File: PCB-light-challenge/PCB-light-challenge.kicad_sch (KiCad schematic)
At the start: 2 parts

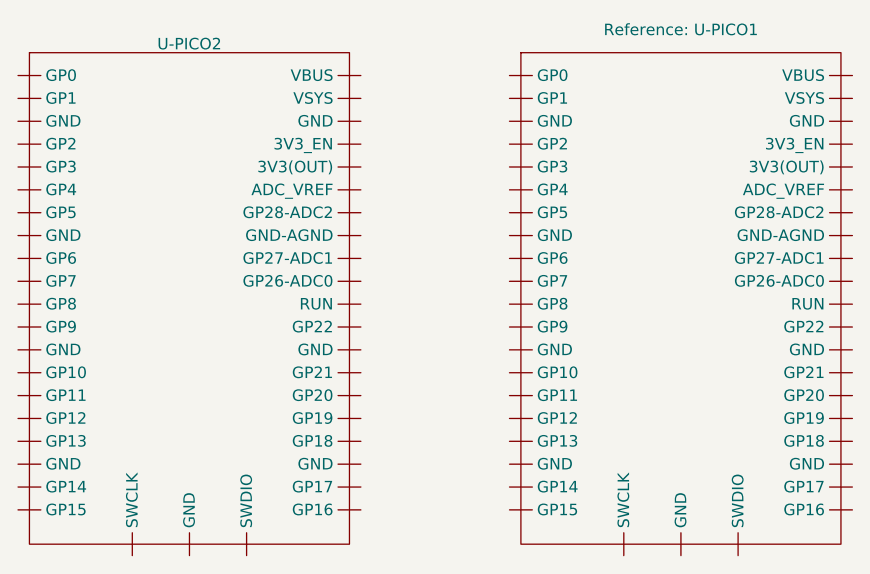
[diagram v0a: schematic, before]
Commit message: Opnieuw
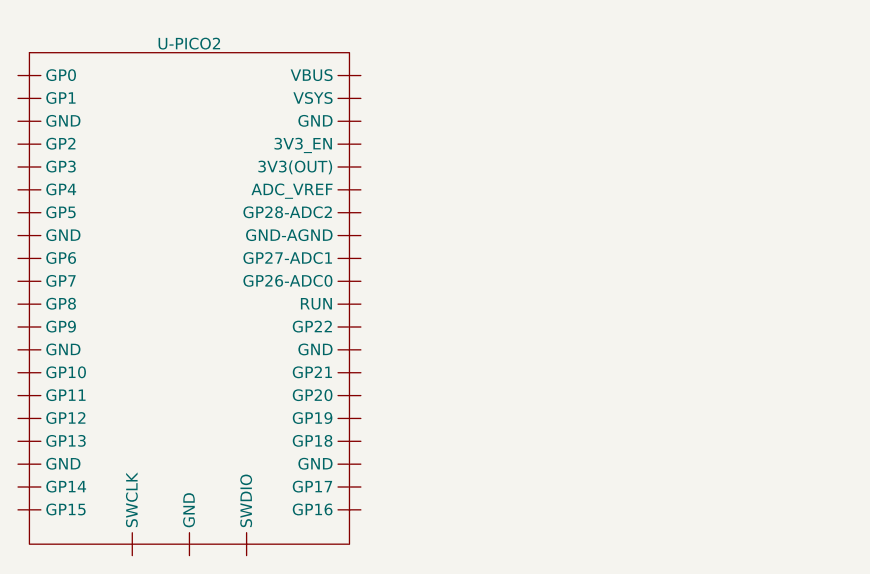
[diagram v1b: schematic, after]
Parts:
- removed U-PICO1: ~, symbol Light_challenge:Raspeberry_Pico
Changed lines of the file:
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@@
-    )
-  )
-  (symbol (lib_id "Light_challenge:Raspeberry_Pico") (at 127 81.28 0) (unit 1)
-    (in_bom yes) (on_board yes) (dnp no) (fields_autoplaced)
-    (property "Reference" "U-PICO1" (at 142.24 77.47 0) (show_name)
-      (effects (font (size 1.27 1.27)))
-    )
-    (property "Value" "~" (at 127 81.28 0) (show_name)
-      (effects (font (size 1.27 1.27)))
-    )
-    (property "Footprint" "" (at 127 81.28 0)
-      (effects (font (size 1.27 1.27)) hide)
-    )
-    (property "Datasheet" "" (at 127 81.28 0)
-      (effects (font (size 1.27 1.27)) hide)
-    )
-    (pin "")
-    (pin "")
-    (pin "")
-    (pin "")
-    (pin "")
-    (pin "")
-    (pin "")
-    (pin "")
-    (pin "")
-    (pin "")
-    (pin "")
-    (pin "")
-    (pin "")
-    (pin "")
-    (pin "")
-    (pin "")
-    (pin "")
-    (pin "")
-    (pin "")
-    (pin "")
-    (pin "")
-    (pin "")
-    (pin "")
-    (pin "")
-    (pin "")
-    (pin "")
-    (pin "")
-    (pin "")
-    (pin "")
-    (pin "")
-    (pin "")
-    (pin "")
-    (pin "")
-    (pin "")
-    (pin "")
-    (pin "")
-    (pin "")
-    (pin "")
-    (pin "")
-    (pin "")
-    (pin "")
-    (pin "")
-    (pin "")
-    (instances
-      (project "PCB-light-challenge"
-        (path "/35573e8f-7834-430c-81d2-239f316c7834"
-          (reference "U-PICO1") (unit 1)
-        )
-      )
     )
   )
